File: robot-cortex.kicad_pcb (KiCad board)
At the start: 4 copper layers, 27.5 x 35.8 mm, 91 parts, among them IC1 THVD2410VDRCR, IC2 THVD2410VDRCR, IC3 THVD2410VDRCR, J1 USB4110GFA, M1 THRU_HOLE_PAD, M2 THRU_HOLE_PAD, Q1 SSM3K15F,LF, Q2 SS8050-G, U1 C2901617, U10 TPS63070, U11 TPS63070, U12 DF52-4S-0.8H(21), U13 DF52-4S-0.8H(21), U14 DF52-4S-0.8H(21), U2 STM32G431CBT6, U3 TLE9250XSJXUMA1, U4 DF52-3S-0.8H(21), U5 DF52-4S-0.8H(21), U6 SPX3819M5-L-5-0, U7 DF52-8S-0.8H(21), U8 ESP32-WROOM-32E-H4, U9 CP2102N-A02-GQFN24R

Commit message: more bom
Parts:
- Q2: value SS8050-G -> SSM3K15F,LF
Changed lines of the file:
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@@
         (effects (font (size 1 1) (thickness 0.15)) (justify mirror))
     )
-    (fp_text value "SS8050-G" (at 0 -2.4 90) (layer "B.Fab") hide
+    (fp_text value "SSM3K15F,LF" (at 0 -2.4 90) (layer "B.Fab") hide
         (effects (font (size 1 1) (thickness 0.15)) (justify mirror))
     )

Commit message: final bom cleanup
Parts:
- L1, L2: value 1277AS-H-1R0M=P2 -> 1uH
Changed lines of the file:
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@@
     (descr "Inductor SMD 1210 (3225 Metric), square (rectangular) end terminal, IPC_7351 nominal, (Body size source: http://www.tortai-tech.com/upload/download/2011102023233369053.pdf), generated with kicad-footprint-generator")
     (tags "inductor")
-    (property "MPN" "ETQ-P3M3R3KVP")
+    (property "DCR" "45mOhm")
+    (property "MPN" "1277AS-H-1R0M=P2")
     (property "Sheetfile" "PSU_TPS63070RNMR.kicad_sch")
     (property "Sheetname" "PSU_TPS63070RNMR")
@@
         (effects (font (size 1 1) (thickness 0.15)))
     )
-    (fp_text value "1277AS-H-1R0M=P2" (at 0.14 -0.655 90) (layer "F.Fab")
+    (fp_text value "1uH" (at 0.14 -0.655 90) (layer "F.Fab")
         (effects (font (size 0.2 0.2) (thickness 0.05)))
     )
@@
     (descr "Inductor SMD 1210 (3225 Metric), square (rectangular) end terminal, IPC_7351 nominal, (Body size source: http://www.tortai-tech.com/upload/download/2011102023233369053.pdf), generated with kicad-footprint-generator")
     (tags "inductor")
-    (property "MPN" "ETQ-P3M3R3KVP")
+    (property "DCR" "45mOhm")
+    (property "MPN" "1277AS-H-1R0M=P2")
     (property "Sheetfile" "PSU_TPS63070RNMR.kicad_sch")
     (property "Sheetname" "PSU_TPS63070RNMR1")
@@
         (effects (font (size 1 1) (thickness 0.15)))
     )
-    (fp_text value "1277AS-H-1R0M=P2" (at 0.14 -0.655) (layer "F.Fab")
+    (fp_text value "1uH" (at 0.14 -0.655) (layer "F.Fab")
         (effects (font (size 0.2 0.2) (thickness 0.05)))
     )

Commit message: found better part
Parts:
- IC1, IC2, IC3: value THVD2410VDRCR -> THVD2450VDRCR
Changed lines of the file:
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@@
     (property "Height" "1")
     (property "Manufacturer_Name" "Texas Instruments")
-    (property "Manufacturer_Part_Number" "THVD2410VDRCR")
+    (property "Manufacturer_Part_Number" "THVD2450VDRCR")
     (property "Mouser Part Number" "595-THVD2410VDRCR")
     (property "Mouser Price/Stock" "https://www.mouser.co.uk/ProductDetail/Texas-Instruments/THVD2410VDRCR?qs=Jm2GQyTW%2FbhjNqkbRGOzgg%3D%3D")
@@
         (effects (font (size 1.27 1.27) (thickness 0.15)) (justify mirror))
     )
-    (fp_text value "THVD2410VDRCR" (at 0 -2.54 90) (layer "B.SilkS") hide
+    (fp_text value "THVD2450VDRCR" (at 0 -2.54 90) (layer "B.SilkS") hide
         (effects (font (size 1.27 1.27) (thickness 0.15)) (justify mirror))
     )
@@
     (property "Height" "1")
     (property "Manufacturer_Name" "Texas Instruments")
-    (property "Manufacturer_Part_Number" "THVD2410VDRCR")
+    (property "Manufacturer_Part_Number" "THVD2450VDRCR")
     (property "Mouser Part Number" "595-THVD2410VDRCR")
     (property "Mouser Price/Stock" "https://www.mouser.co.uk/ProductDetail/Texas-Instruments/THVD2410VDRCR?qs=Jm2GQyTW%2FbhjNqkbRGOzgg%3D%3D")
@@
         (effects (font (size 1.27 1.27) (thickness 0.15)) (justify mirror))
     )
-    (fp_text value "THVD2410VDRCR" (at 0 -2.54 90) (layer "B.SilkS") hide
+    (fp_text value "THVD2450VDRCR" (at 0 -2.54 90) (layer "B.SilkS") hide
         (effects (font (size 1.27 1.27) (thickness 0.15)) (justify mirror))
     )
@@
     (property "Height" "1")
     (property "Manufacturer_Name" "Texas Instruments")
-    (property "Manufacturer_Part_Number" "THVD2410VDRCR")
+    (property "Manufacturer_Part_Number" "THVD2450VDRCR")
     (property "Mouser Part Number" "595-THVD2410VDRCR")
     (property "Mouser Price/Stock" "https://www.mouser.co.uk/ProductDetail/Texas-Instruments/THVD2410VDRCR?qs=Jm2GQyTW%2FbhjNqkbRGOzgg%3D%3D")
@@
         (effects (font (size 1.27 1.27) (thickness 0.15)) (justify mirror))
     )
-    (fp_text value "THVD2410VDRCR" (at 0 -2.54 90) (layer "B.SilkS") hide
+    (fp_text value "THVD2450VDRCR" (at 0 -2.54 90) (layer "B.SilkS") hide
         (effects (font (size 1.27 1.27) (thickness 0.15)) (justify mirror))
     )

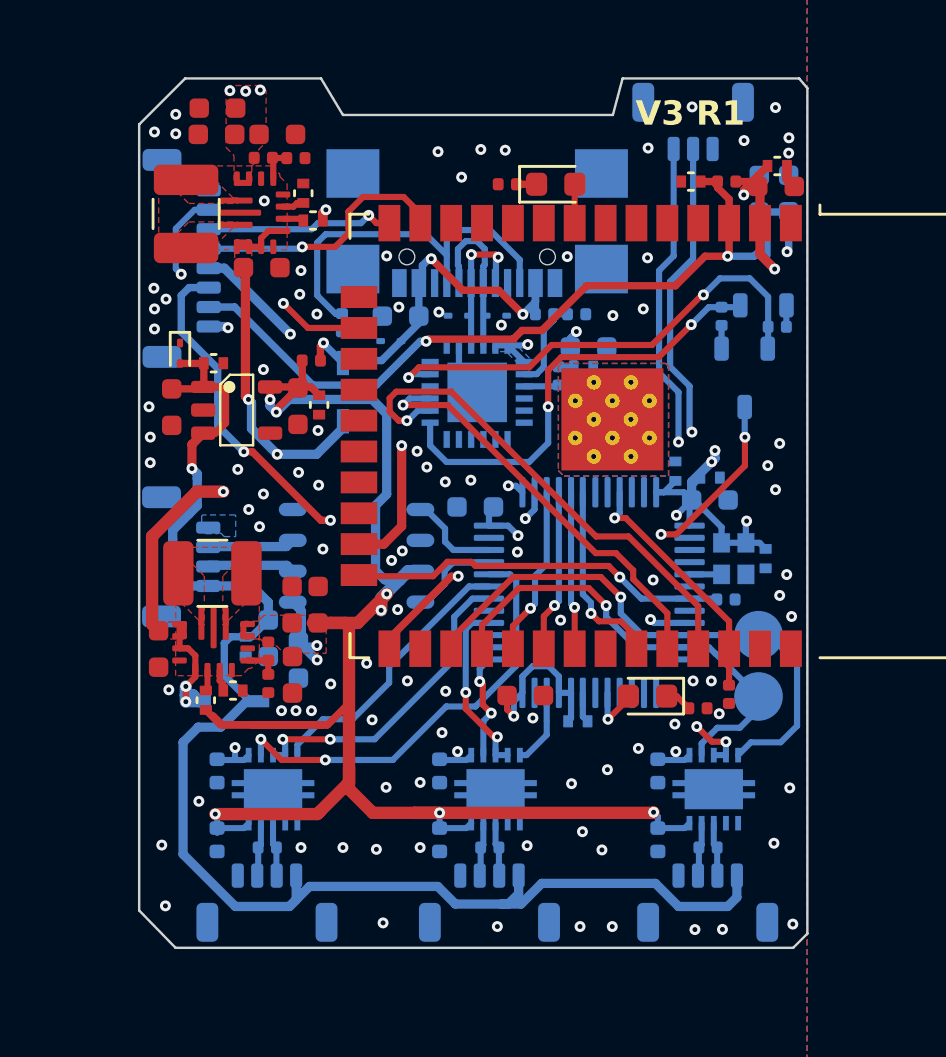
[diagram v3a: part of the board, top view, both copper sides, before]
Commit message: curvy
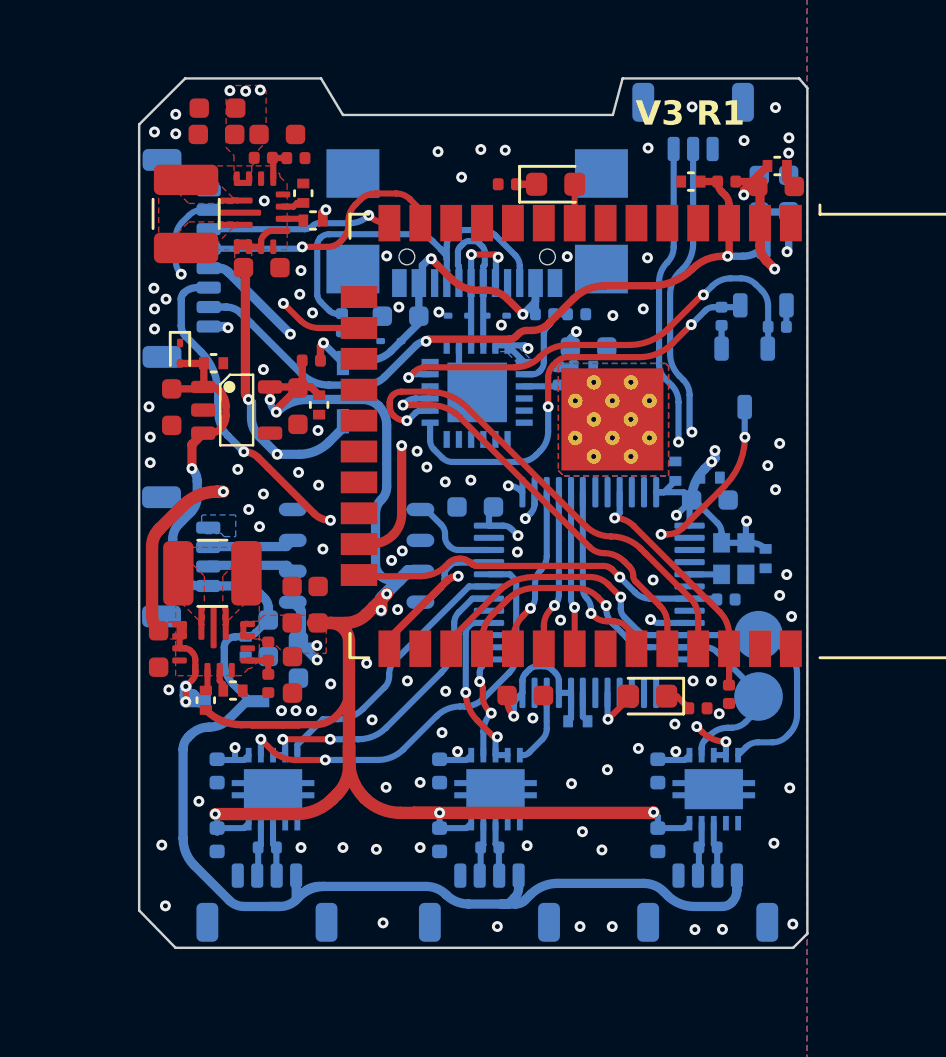
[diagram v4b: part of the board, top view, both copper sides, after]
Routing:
- net /+5V0: track 76.9 -> 70.4 mm
- net +3V3: track 55.5 -> 53.9 mm
- net /ESP32/IO0: track 40.1 -> 39.3 mm
- net /ESP32/EN: track 30.5 -> 29.8 mm
- net /VDD_MIXED: track 29.8 -> 29.3 mm
